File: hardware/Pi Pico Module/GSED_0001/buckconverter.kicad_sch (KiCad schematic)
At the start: 10 parts, among them U2 LMR33640ADDAR

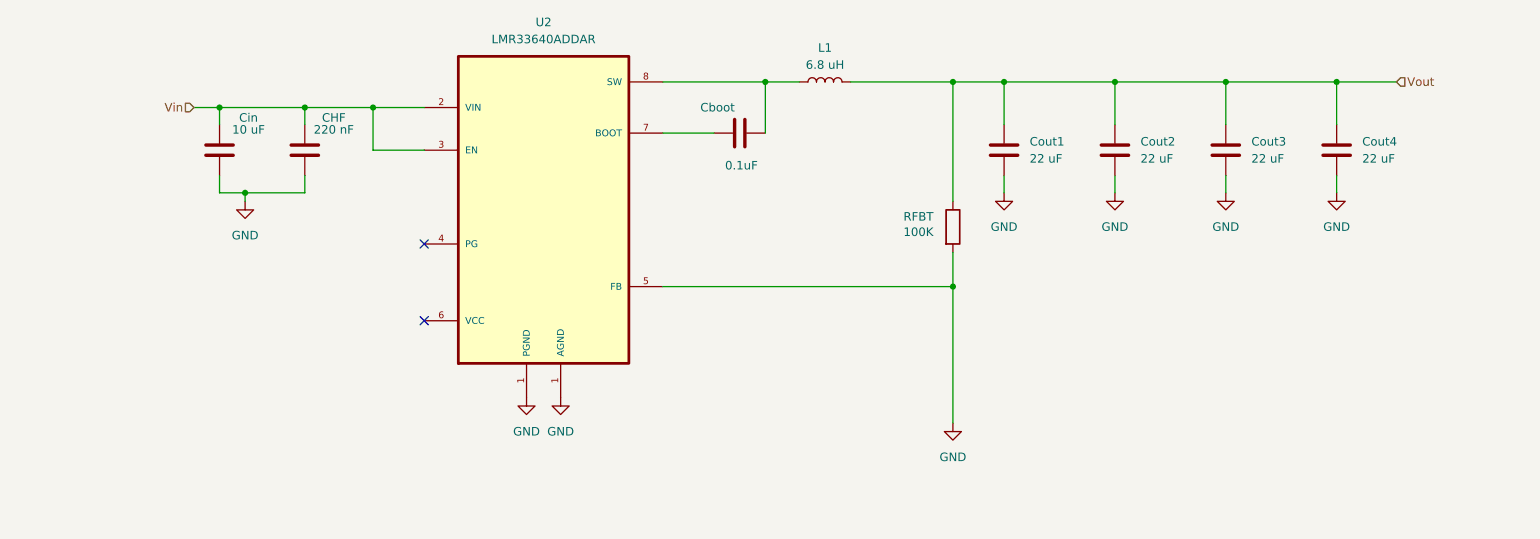
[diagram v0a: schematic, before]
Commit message: Reuploaded folder
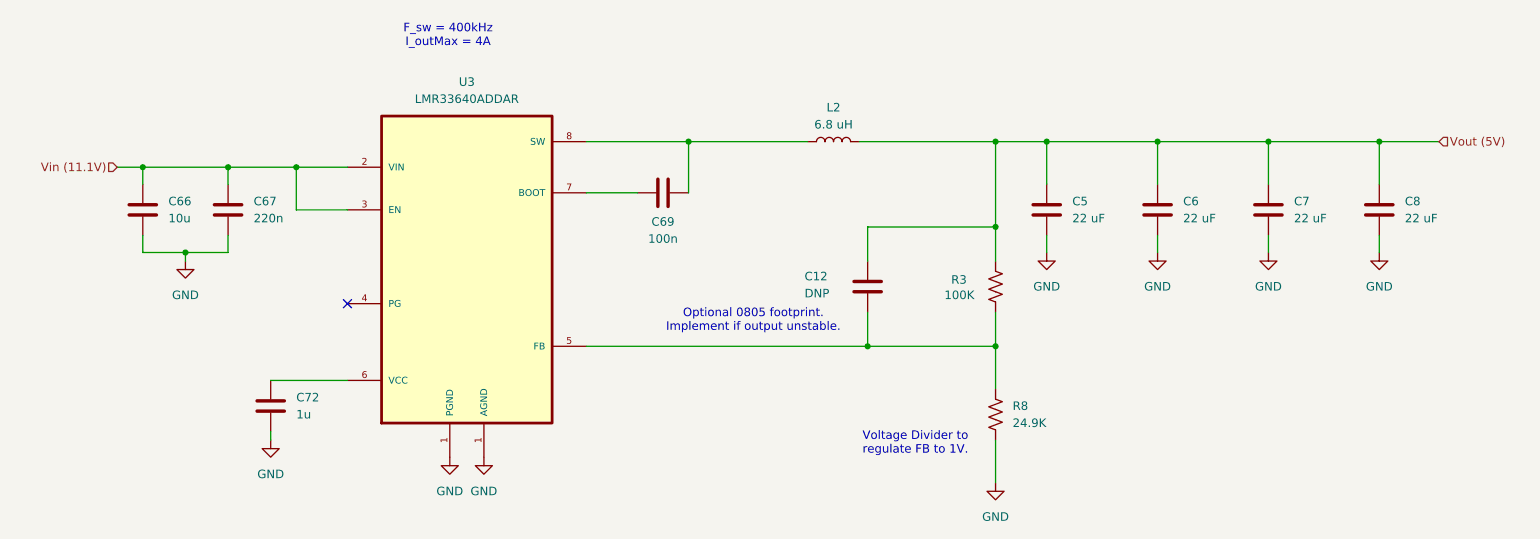
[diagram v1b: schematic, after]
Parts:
- removed CHF: 220 nF, symbol Device:C
- removed Cboot: 0.1uF, symbol Device:C
- removed Cin: 10 uF, symbol Device:C
- removed Cout2, Cout3, Cout4: 22 uF, symbol Device:C
- removed L1: 6.8 uH, symbol Device:L
- removed RFBT: 100K, symbol Device:R
- removed U2: LMR33640ADDAR, LMR33640ADDAR:VREG_LM5017MR_NOPB, symbol LMR33640ADDAR:LMR33640ADDAR
- added C12: DNP, Capacitor_SMD:C_0805_2012Metric, symbol Device:C
- added C6, C7, C8: 22 uF, Capacitor_SMD:C_0805_2012Metric, symbol Device:C
- added C66: 10u, Capacitor_SMD:C_0805_2012Metric, symbol Device:C
- added C67: 220n, Capacitor_SMD:C_0805_2012Metric, symbol Device:C
- added C69: 100n, Capacitor_SMD:C_0603_1608Metric, symbol Device:C
- added C72: 1u, Capacitor_SMD:C_0805_2012Metric, symbol Device:C
- added L2: 6.8 uH, CSBX0650_6R8M:IND_CSBX0650-6R8M, symbol Device:L
- added R3: 100K, Resistor_SMD:R_0603_1608Metric, symbol Device:R_US
- added R8: 24.9K, Resistor_SMD:R_0603_1608Metric, symbol Device:R_US
- added U3: LMR33640ADDAR, LMR33640ADDAR:VREG_LM5017MR_NOPB, symbol LMR33640ADDAR:LMR33640ADDAR
- C5: renamed from Cout1; footprint (none) -> Capacitor_SMD:C_0805_2012Metric; DigiKey (none) -> https://www.digikey.com/en/products/detail/samsung-electro-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
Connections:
- net GND: now also C6.2, C66.2, C67.2, C7.2, C72.2, C8.2, R8.2, U3.1 (AGND)
- net Vout renamed Vout (5V)
- net Vout (5V): now also C12.2, C6.1, C7.1, C8.1, L2.2, R3.2
- new net: C69.2, L2.1, U3.8 (SW)
- new net: C69.1, U3.7 (BOOT)
- new net: C72.1, U3.6 (VCC)
- new net: C12.1, R3.1, R8.1, U3.5 (FB)
- new net Vin (11.1V): C66.1, C67.1, U3.2 (VIN), U3.3 (EN)
- no-connect marks 2 -> 1
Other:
- note added: "F_sw = 400kHz I_outMax = 4A"
- note added: "Optional 0805 footprint. Implement if output unstable."
- note added: "Voltage Divider to regulate FB to 1V."
- moved on the sheet: C5
